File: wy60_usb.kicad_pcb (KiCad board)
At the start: 2 copper layers, 409.1 x 170.9 mm, 223 parts, among them J1 AVR-ISP-6, U1 ATmega32A-PU

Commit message: rev2
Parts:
- moved C3 8.89 mm to (256.9, 69.1)
- moved G*** 7.15 mm to (125.0, 63.5)
- moved G*** 7.15 mm to (147.7, 63.4)
- moved R4 4.64 mm to (326.9, 70.1)
- moved Boot1 4.51 mm to (325.4, 60.3)
- moved Reset1 4.51 mm to (312.4, 60.3)
- moved C1 3.82 mm to (72.5, 67.3)
- moved D1 3.82 mm to (99.9, 67.4)
- moved D2 3.82 mm to (103.5, 67.4)
- moved F1 3.82 mm to (63.6, 67.3)
- moved R1 3.82 mm to (86.6, 68.6)
- moved R2 3.82 mm to (91.2, 68.6)
- moved R3 3.82 mm to (95.5, 68.6)
- moved C2 2.92 mm to (259.3, 53.7)
- moved C5 2.80 mm to (286.8, 56.8)
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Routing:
- net +5V: track 359.7 -> 347.4 mm
- net col15: track 139.2 -> 146.7 mm
- net row3: track 475.3 -> 481.5 mm
- net row4: track 489.1 -> 495.2 mm
- net row1: track 450.1 -> 455.9 mm
- net row5: track 532.5 -> 537.3 mm
- net row2: track 460.0 -> 464.6 mm
- net col2: track 313.7 -> 309.7 mm
- net col1: track 347.9 -> 344.2 mm
- net col4: track 286.7 -> 283.4 mm
- net col3: track 303.0 -> 299.8 mm
- net col14: track 134.4 -> 137.6 mm
- net col11: track 131.6 -> 134.8 mm
- net col7: track 249.6 -> 246.5 mm
- net col6: track 250.3 -> 247.5 mm
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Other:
- board size 409.1 x 170.9 mm -> 407.9 x 170.4 mm
- board text added: "WY-60 USB PCB rev. 2 github.com/kb-elmo/wy60_usb elmo.space"
- board text removed: "WY-60 USB PCB rev. 1 github.com/kb-elmo/wy60_usb elmo.space"

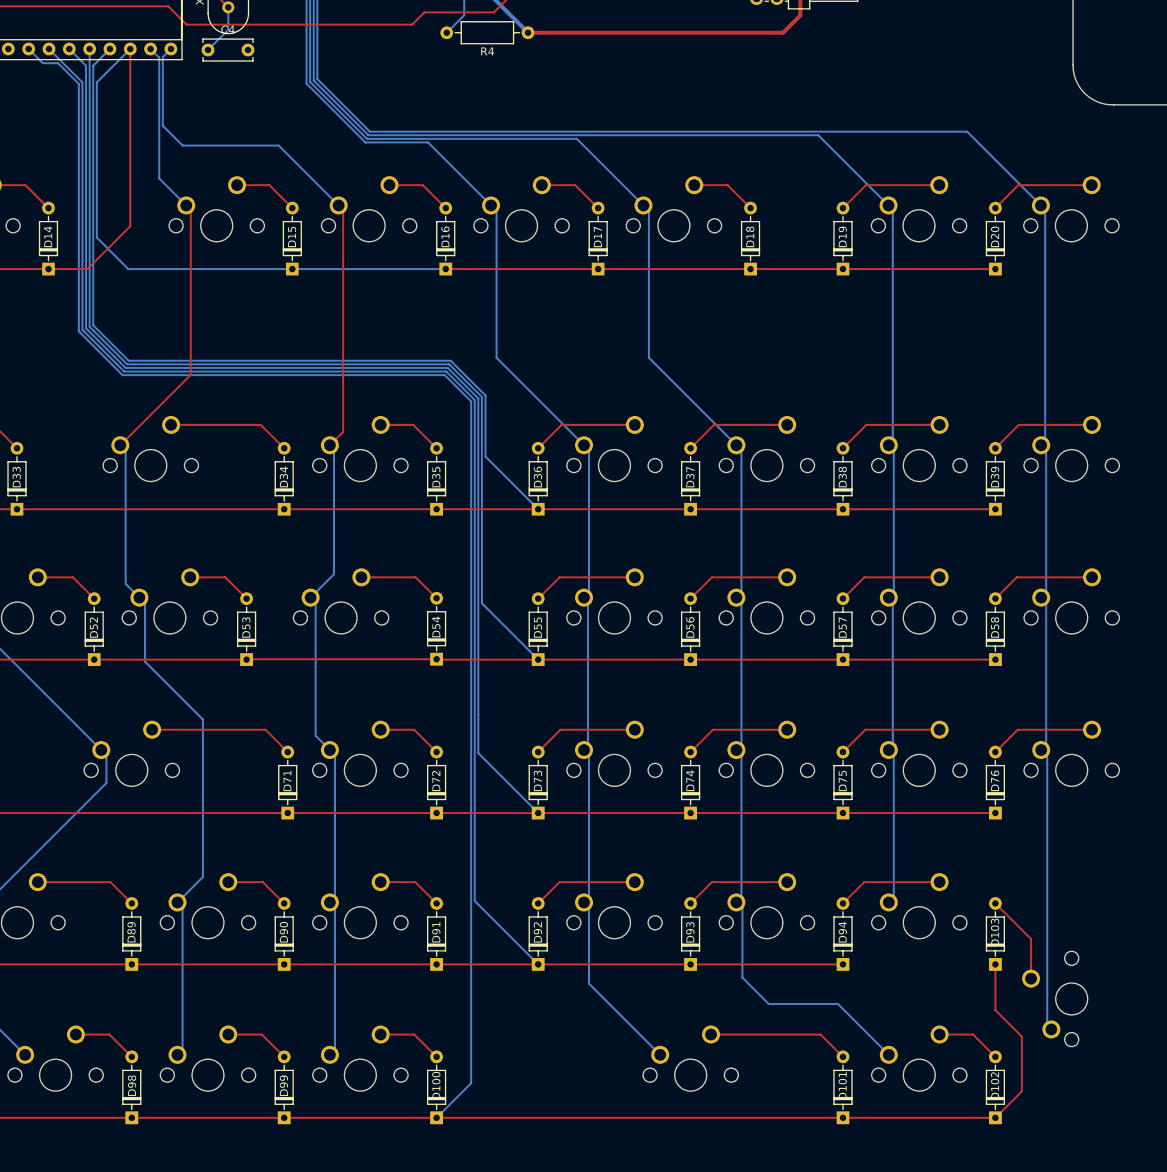
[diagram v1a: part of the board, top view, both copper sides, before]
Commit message: fixed spacing
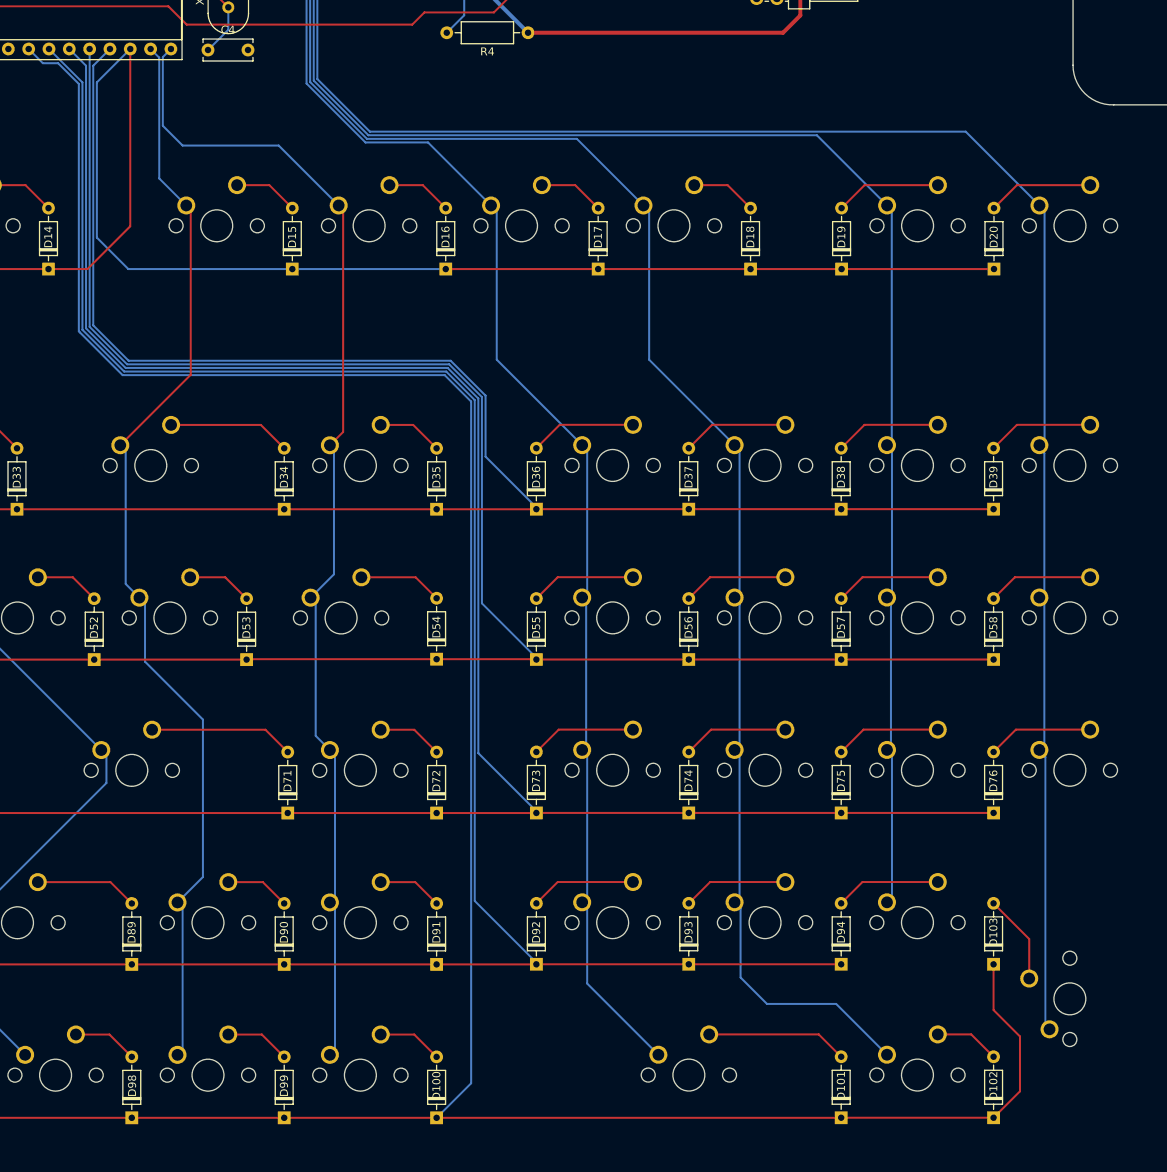
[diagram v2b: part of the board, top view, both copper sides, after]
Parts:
- moved MX71 0.23 mm to (337.5, 162.3)
- moved MX72 0.23 mm to (356.5, 162.3)
- moved MX34 0.23 mm to (337.5, 124.2)
- moved MX35 0.23 mm to (356.5, 124.2)
- moved D36 0.23 mm to (327.9, 129.7)
- moved D37 0.23 mm to (347.0, 129.7)
- moved D55 0.23 mm to (327.9, 148.5)
- moved D56 0.23 mm to (347.0, 148.5)
- moved D73 0.23 mm to (327.9, 167.6)
- moved D74 0.23 mm to (347.0, 167.6)
- moved D92 0.23 mm to (327.9, 186.6)
- moved D93 0.23 mm to (347.0, 186.6)
- moved MX53 0.23 mm to (337.5, 143.2)
- moved MX54 0.23 mm to (356.5, 143.2)
- moved MX90 0.23 mm to (337.5, 181.3)
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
